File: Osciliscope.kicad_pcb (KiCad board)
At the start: 2 copper layers, 51 x 102 mm, 62 parts, among them J1 Conn_01x09_Socket, J2 Conn_01x04_Socket, J3 U.FL, J4 Conn_01x04_Socket, J5 USB_C_Receptacle_USB2.0_14P, J6 Conn_01x02_MountingPin, J7 U.FL, SW1 RotaryEncoder_Switch, SW3 SW_Nidec_CAS-120A1, SW4 SW_Nidec_CAS-120A1, SW5 RotaryEncoder_Switch, SW6 RotaryEncoder_Switch, U1 MCP1700x-330xxMB, U2 ADC082S101, U3 IP2721, U4 AZ1084-5.0, U5 TLV9061xDBV, U7 TLV9061xDBV, U8 MCP4251-104E/ML-ND

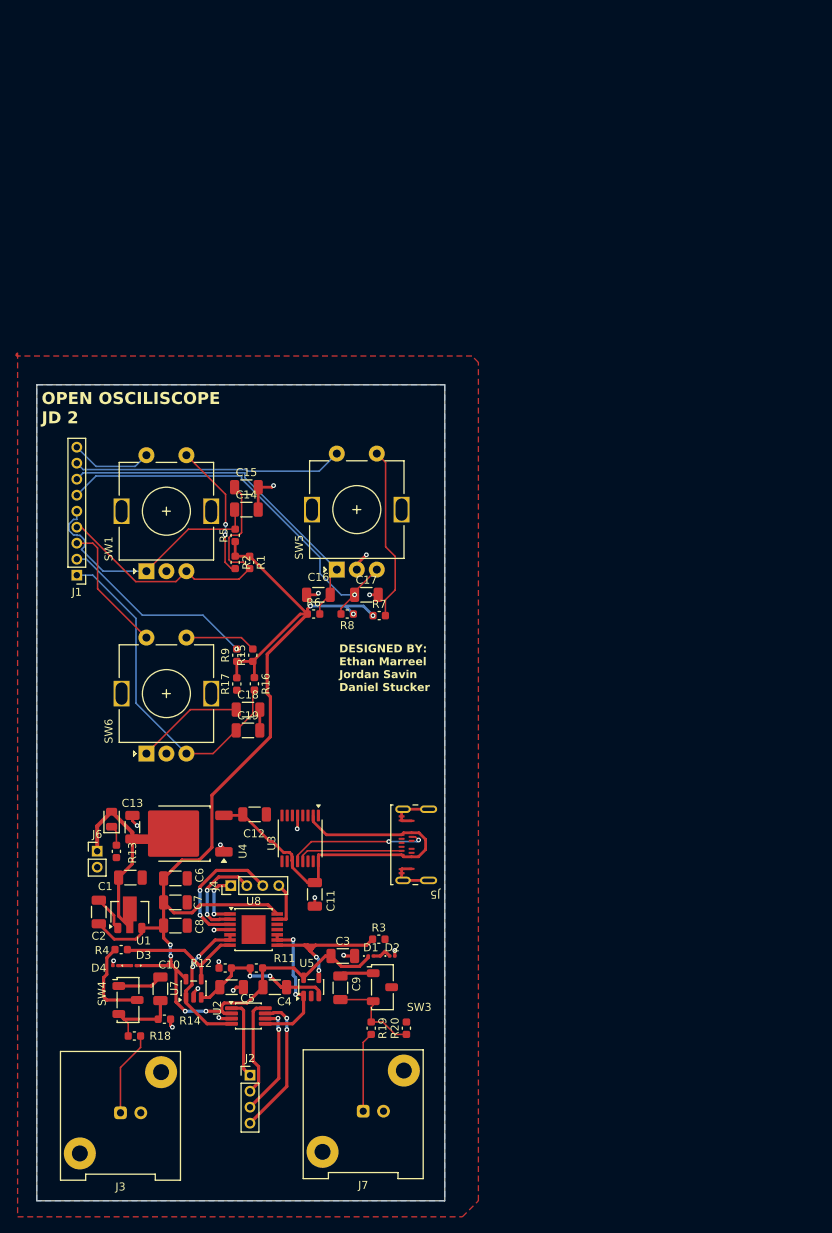
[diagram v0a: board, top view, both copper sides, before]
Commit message: DOUBLE POWAH
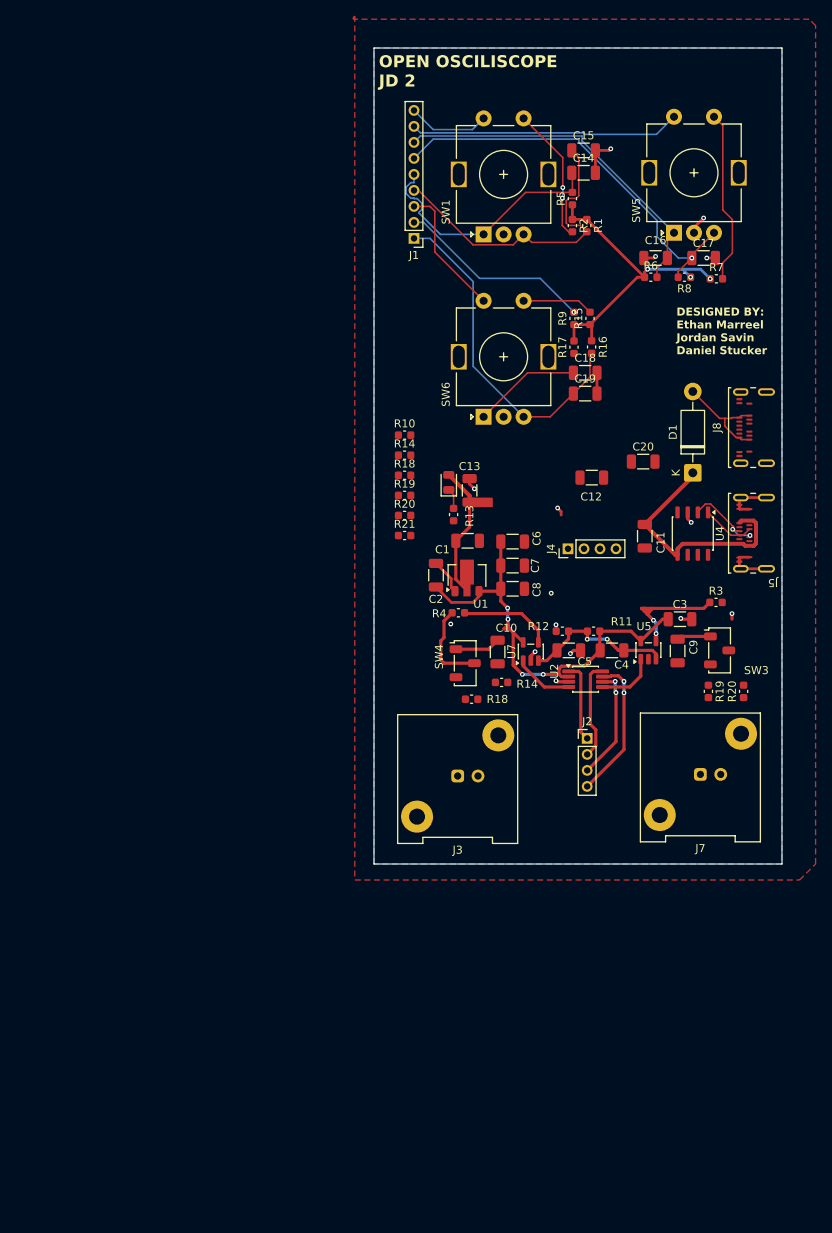
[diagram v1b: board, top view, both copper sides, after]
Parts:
- removed D2, D3, D4: D, Diode_SMD:D_0201_0603Metric
- removed J6: Conn_01x02_MountingPin, Connector_PinHeader_2.00mm:PinHeader_1x02_P2.00mm_Vertical
- removed U3: IP2721, Package_SO:TSSOP-16_4.4x5mm_P0.65mm
- removed U8: MCP4251-104E/ML-ND, Package_SO:TSSOP-14-1EP_4.4x5mm_P0.65mm
- added C20: 20pF, Capacitor_SMD:C_1206_3216Metric, F.Cu at (145.8, 99.6)
- added J8: USB_C_Receptacle_USB2.0_14P, Connector_USB:USB_C_Receptacle_Amphenol_124019772112A, F.Cu at (161.0, 95.3)
- added R10: 10k, Capacitor_SMD:C_0603_1608Metric, F.Cu at (116.0, 96.3)
- added R14: 1M, Capacitor_SMD:C_0603_1608Metric, F.Cu at (116.0, 98.8)
- added R18: 10k, Capacitor_SMD:C_0603_1608Metric, F.Cu at (116.0, 101.3)
- added R19: 1M, Capacitor_SMD:C_0603_1608Metric, F.Cu at (116.0, 103.8)
- added R20: 1M, Capacitor_SMD:C_0603_1608Metric, F.Cu at (116.0, 106.3)
- added R21: 1M, Capacitor_SMD:C_0603_1608Metric, F.Cu at (116.0, 108.8)
- C11: value 1uF -> 100n
- C12: value 10u -> 100n
- D1: value D -> 1N4001; footprint Diode_SMD:D_0201_0603Metric -> Diode_THT:D_DO-41_SOD81_P10.16mm_Horizontal
- R14, R20: value 100k -> 1M
- R18: value 1M -> 10k
- R3, R4: value 5k -> 10k
- U4: value AZ1084-5.0 -> CH340N; footprint Package_TO_SOT_SMD:TO-252-2 -> Package_SO:JEITA_SOIC-8_3.9x4.9mm_P1.27mm
- moved U4 73.9 mm to (152.0, 108.6), turned to -90 degrees
- moved D1 72.6 mm to (152.0, 101.0), turned to 90 degrees
- moved C11 60.9 mm to (146.0, 108.9)
- moved J2 59.6 mm to (138.8, 134.2)
- moved C2 59.6 mm to (119.9, 113.8)
- moved C3 59.6 mm to (150.4, 119.3)
- moved C4 59.6 mm to (141.9, 123.2)
- moved C5 59.6 mm to (136.5, 123.2)
- moved D5 59.6 mm to (121.5, 102.2)
- moved R1 59.6 mm to (138.8, 70.1)
- moved R17 59.6 mm to (137.2, 85.3)
- moved R3 59.6 mm to (154.9, 117.2)
- moved R6 59.6 mm to (146.8, 76.5)
- moved J7 59.6 mm to (152.9, 138.7)
- moved R19 59.6 mm to (153.9, 128.3)
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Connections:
- net C2_G_IN renamed Net-(U7--)
- net C2_G_OUT renamed CHAN_2
- C10 pad 1: Net-(SW4-A) -> Net-(J3-In)
- C11 pad 1: USBCRAW -> 5Vin
- C12 pad 1: USBCRAW -> Net-(U4-V3)
- C9 pad 1: Net-(SW3-A) -> Net-(J7-In)
- D1 pad 1: V3.3 -> 5Vin
- J5 pad A4: USBCRAW -> 5Vin
- J5 pad A6: unconnected-(J5-D+-PadA6) -> Net-(U4-UD+)
- J5 pad A7: unconnected-(J5-D--PadA7) -> Net-(U4-UD-)
- J5 pad A9: USBCRAW -> 5Vin
- J5 pad B4: USBCRAW -> 5Vin
- J5 pad B6: unconnected-(J5-D+-PadB6) -> Net-(U4-UD+)
- J5 pad B7: unconnected-(J5-D--PadB7) -> Net-(U4-UD-)
- J5 pad B9: USBCRAW -> 5Vin
- R14 pad 1: Net-(SW4-A) -> GND
- R14 pad 2: GND -> Net-(J3-In)
- R18 pad 1: Net-(SW4-A) -> CHAN_1
- R18 pad 2: Net-(J3-In) -> Net-(U5--)
- R19 pad 1: Net-(SW3-A) -> Net-(J7-In)
- R19 pad 2: Net-(J7-In) -> Net-(SW3-C)
- R20 pad 1: Net-(SW3-A) -> GND
- R20 pad 2: GND -> Net-(J7-In)
- R3 pad 1: C1_G_IN -> Net-(U5--)
- R3 pad 2: unconnected-(R3-Pad2) -> Net-(SW3-B)
- SW3 pad 2: unconnected-(SW3-B-Pad2) -> Net-(SW3-B)
- SW3 pad 3: Net-(SW3-A) -> Net-(J7-In)
- SW4 pad 3: Net-(SW4-A) -> Net-(J3-In)
- U2 pad 5: C1_G_OUT -> CHAN_1
- U4 pad 1: GND -> Net-(U4-UD+)
- U4 pad 2: 5Vin -> Net-(U4-UD-)
- U4 pad 3: USBCRAW -> GND
- U5 pad 1: C1_G_OUT -> CHAN_1
- U5 pad 4: C1_G_IN -> Net-(U5--)
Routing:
- net V3.3: track 163.7 -> 96.4 mm
- net USBCRAW: track 51.3 -> 0.00 mm
- net 5Vin: track 22.5 -> 47.3 mm
- net C1_G_IN: track 19.2 -> 0.00 mm, vias 2 -> 0
- net C1_G_OUT: track 18.2 -> 0.00 mm, vias 2 -> 0
- net Net-(J5-CC2): track 17.7 -> 0.00 mm, vias 2 -> 0
- net RPI_DIN_DP: track 17.3 -> 0.00 mm, vias 2 -> 0
- net Net-(U5--): track 0.00 -> 15.8 mm, vias 0 -> 2
- net Net-(J5-CC1): track 13.3 -> 0.00 mm
- net RPI_SCLK_DP: track 12.4 -> 0.00 mm, vias 2 -> 0
- net Net-(SW3-A): track 11.4 -> 0.00 mm
- net CHAN_2: track 18.6 -> 7.44 mm, vias 2 -> 0
- net Net-(SW4-A): track 10.9 -> 0.00 mm
- net Net-(D1-A): track 2.52 -> 13.4 mm
- net Net-(J3-In): track 10.6 -> 0.00 mm
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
